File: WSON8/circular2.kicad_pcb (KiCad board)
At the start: 2 copper layers, 25 x 25 mm, 32 parts, among them J101 Conn_Coaxial, J102 Conn_01x03, U101 LT3042xMSE, U102 LT3093xMSE, U103 OPA859xDSG, U104 BUF602xDBV

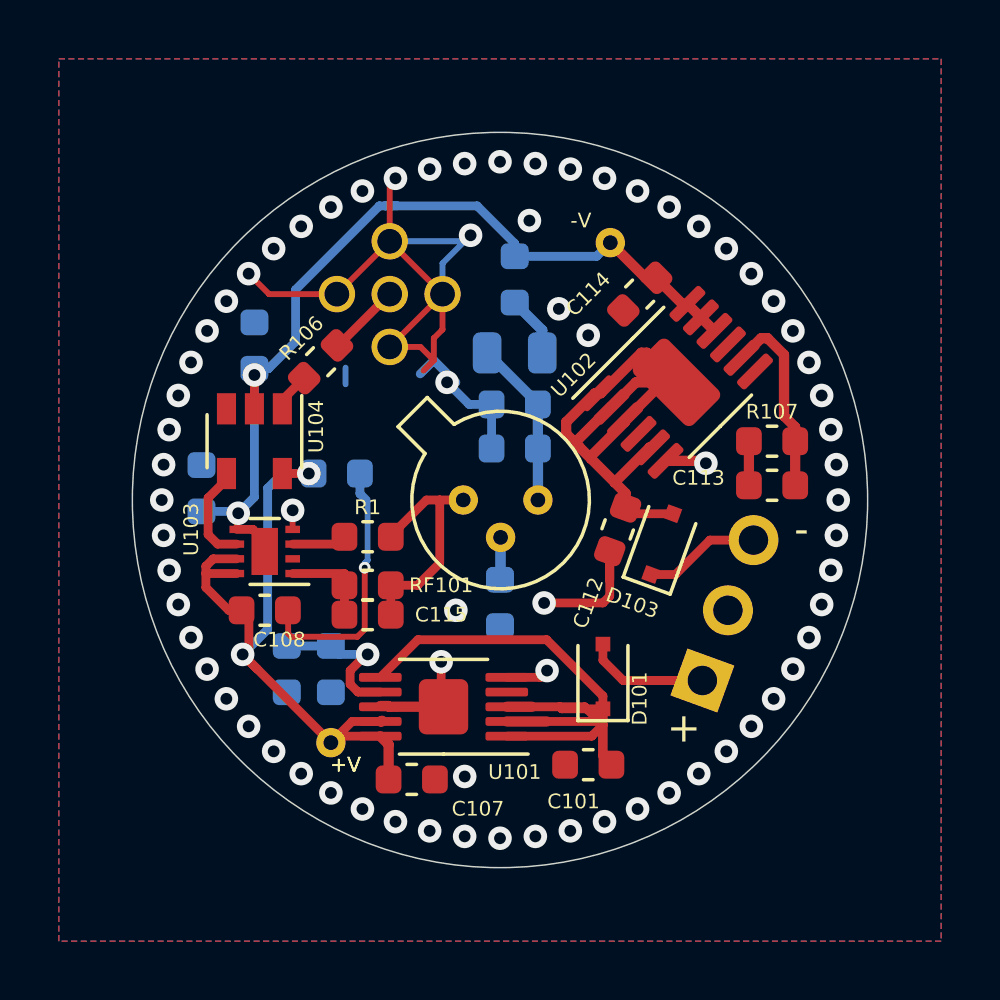
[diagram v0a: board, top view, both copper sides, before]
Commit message: prep for OPA858 build
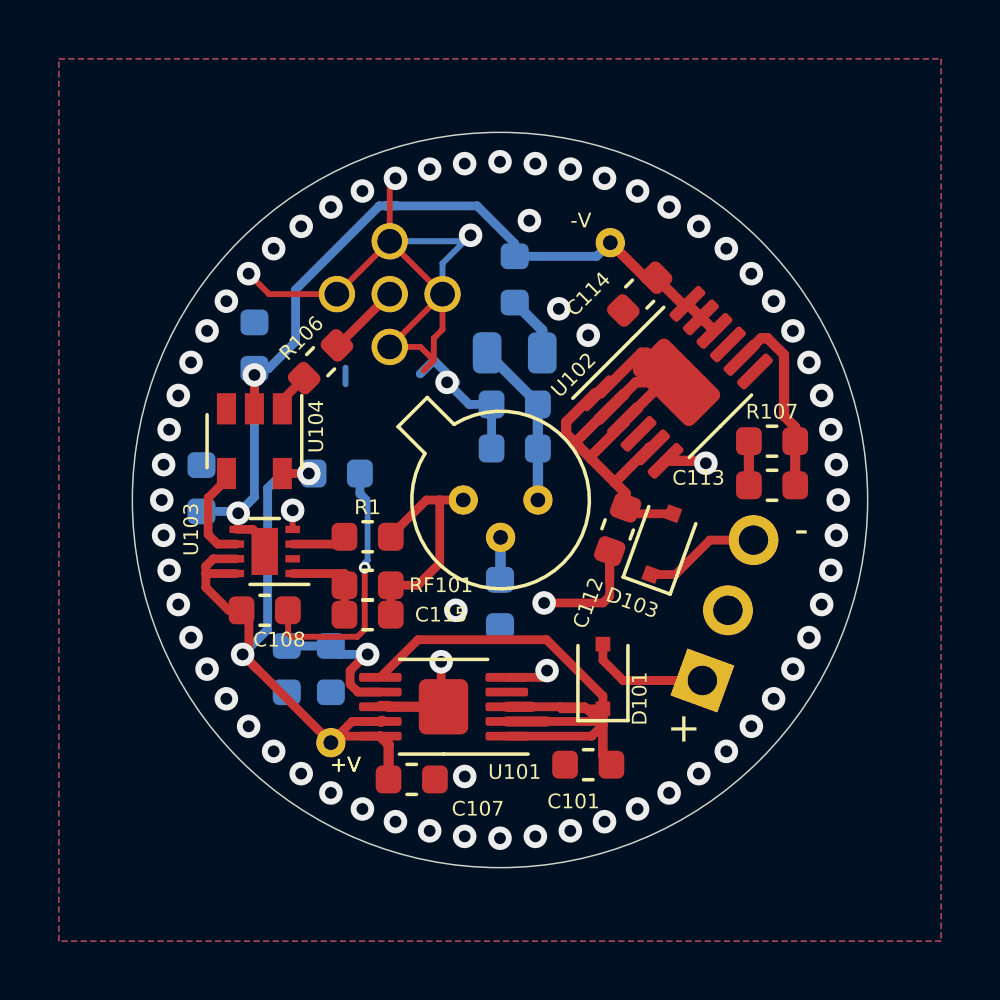
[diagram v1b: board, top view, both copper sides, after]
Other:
- net class Default removed
- net class PWR removed
